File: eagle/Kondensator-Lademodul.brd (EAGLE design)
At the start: 67 x 34.3 mm, 12 parts, among them X1 MKDSN1,5/2-5,08, X2 MKDSN1,5/2-5,08

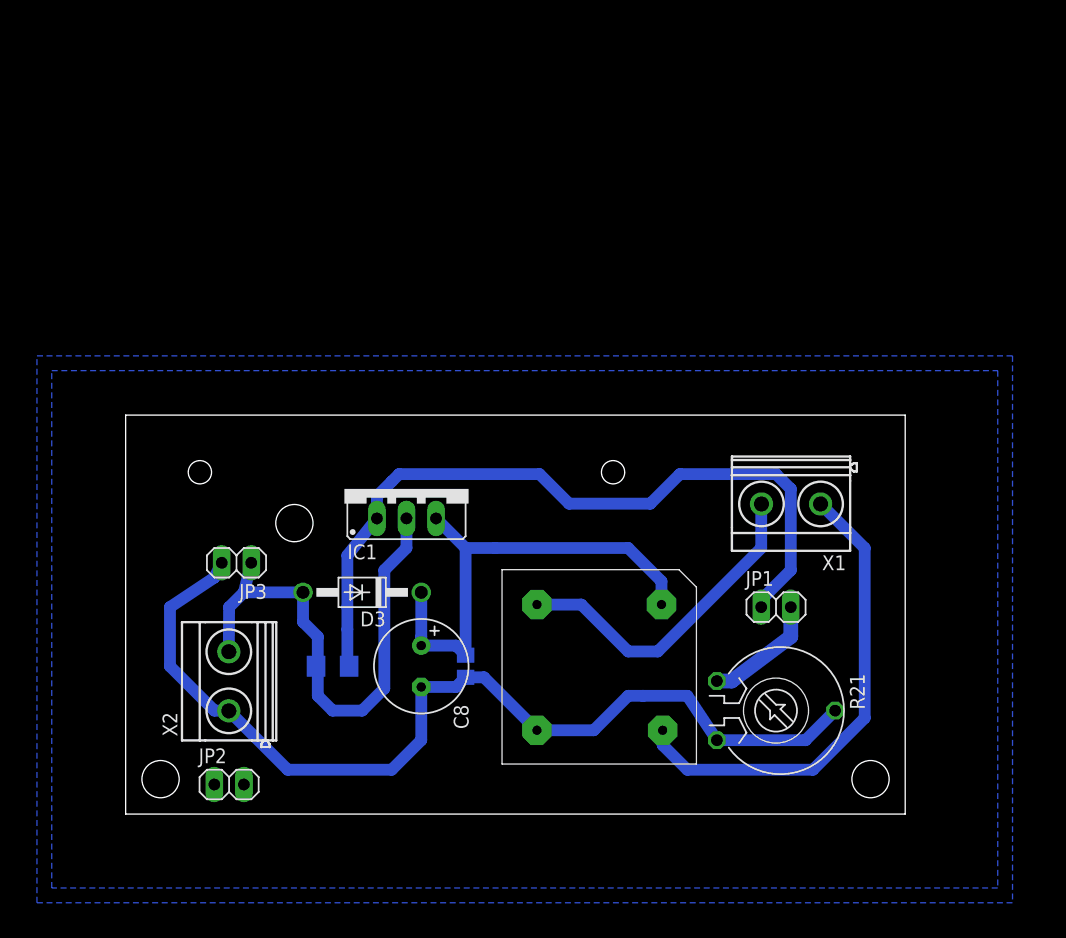
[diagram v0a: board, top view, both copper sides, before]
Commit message: pcb design
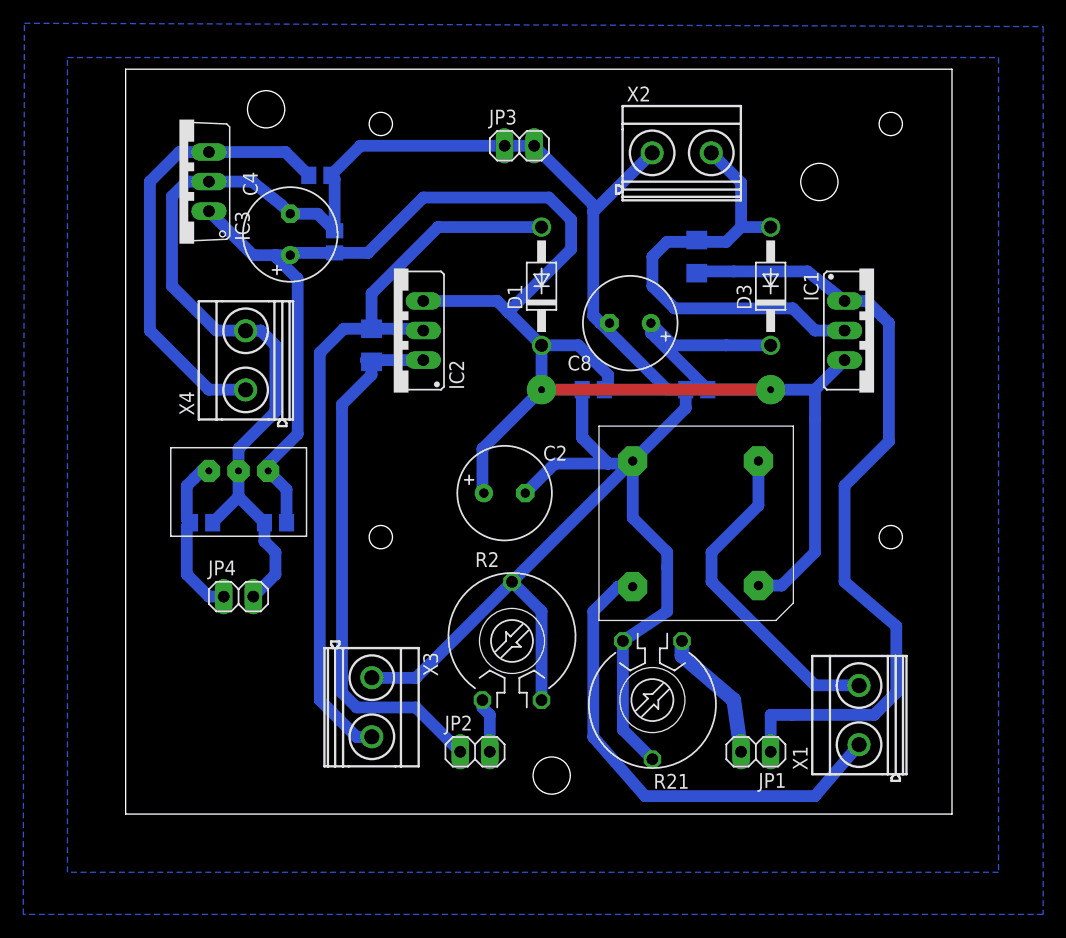
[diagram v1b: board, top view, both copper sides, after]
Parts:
- added C1, C3, C5, C6, C9: 100nF, rcl:C0805
- added C2: 100µ, rcl:E3,5-8
- added C4: 1000µ, rcl:E3,5-8
- added D1: 1N4004, diode:DO41-10
- added IC2: (no value), v-reg:317TS
- added IC3: 7818TV, linear:TO220V
- added JP4: (no value), pinhead:1X02
- added R1: 100k, rcl:R1206
- added R2: (no value), pot:PT-10
- added U$1: DCDC-WANDLER, 0liver:TRACOPOWER-DCDCWANDER-TSR1
- added X3, X4: MKDSN1,5/2-5,08, con-phoenix-508:MKDSN1,5/2-5,08
- moved X2 59.8 mm to (47.8, 56.8), turned to 0 degrees
- moved R20 47.1 mm to (49.1, 47.9), turned to 90 degrees
- moved D3 43.9 mm to (55.4, 45.4), turned to 90 degrees
- moved JP3 43.3 mm to (33.8, 57.4), turned to 0 degrees
- moved IC1 42.4 mm to (64.3, 41.5), turned to 270 degrees
- moved C8 34.5 mm to (43.4, 42.2), turned to 180 degrees
- moved C7 31.0 mm to (49.1, 36.5), turned to 0 degrees
- moved JP2 21.3 mm to (30.0, 5.35)
- moved X1 19.1 mm to (63.0, 8.53), turned to 90 degrees
- moved U$2 14.9 mm to (49.1, 25.0), turned to 180 degrees
- moved JP1 12.5 mm to (54.1, 5.35), turned to 180 degrees
- moved R21 10.7 mm to (45.3, 9.79), turned to 180 degrees
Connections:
- removed net N$27: C7.1, C8.+, D3.C, IC1.3, U$2.+
- new net N$17: C1.1, C2.+, C3.1, C4.+, C5.1, C7.1, C8.+, D1.C, D3.C, IC1.3, IC2.3, IC3.1, U$1.1, U$2.+
- new net N$2: C6.1, IC3.3, X4.1
- new net N$3: D1.A, IC2.2, R1.2, X3.2
- new net N$4: IC2.1, JP2.1, R1.1
- new net N$5: JP2.2, R2.A
- new net N$6: C9.1, JP4.1, U$1.3
- net GND: now also C1.2, C2.-, C3.2, C4.-, C5.2, C6.2, C9.2, IC3.2, JP3.1, JP4.2, R2.E, R2.S, U$1.2, X3.1, X4.2; no longer JP2.2
- net N$28: no longer JP2.1, JP3.1
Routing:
- net N$17: track 0.00 -> 182.7 mm, vias 0 -> 2
- net GND: track 84.1 -> 226.8 mm
- net N$3: track 0.00 -> 65.4 mm
- net N$4: track 0.00 -> 47.2 mm
- net N$27: track 41.5 -> 0.00 mm
- net N$2: track 0.00 -> 38.7 mm
- net N$6: track 0.00 -> 14.3 mm
- net N$28: track 45.3 -> 39.4 mm
- net N$5: track 0.00 -> 4.71 mm
- net N$30: track 65.8 -> 68.5 mm
- net N$29: track 10.2 -> 11.6 mm
- net N$25: track 41.3 -> 42.2 mm
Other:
- board size 67 x 34.3 mm -> 71 x 64 mm
- board text added: "36V ~ IN"
- board text added: "GND"
- board text added: "Poti V1"
- board text added: "Poti V2"
- board text added: "Widerstandskaskade 1"
- board text added: "Widerstandskaskade 2"
